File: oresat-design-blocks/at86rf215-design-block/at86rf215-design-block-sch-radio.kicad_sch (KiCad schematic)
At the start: 40 parts, among them J1 SMA, J2 USB4105-GF-A, J3 Conn_01x04, J5 Conn_02x20_Odd_Even, J6 Conn_01x04, J9 Screw_Terminal_01x02, SW1 RESET, U1 AT86RF215, U2 LP2985AIM5-1.8_NOPB, X1 TXETALSANF-26.000000

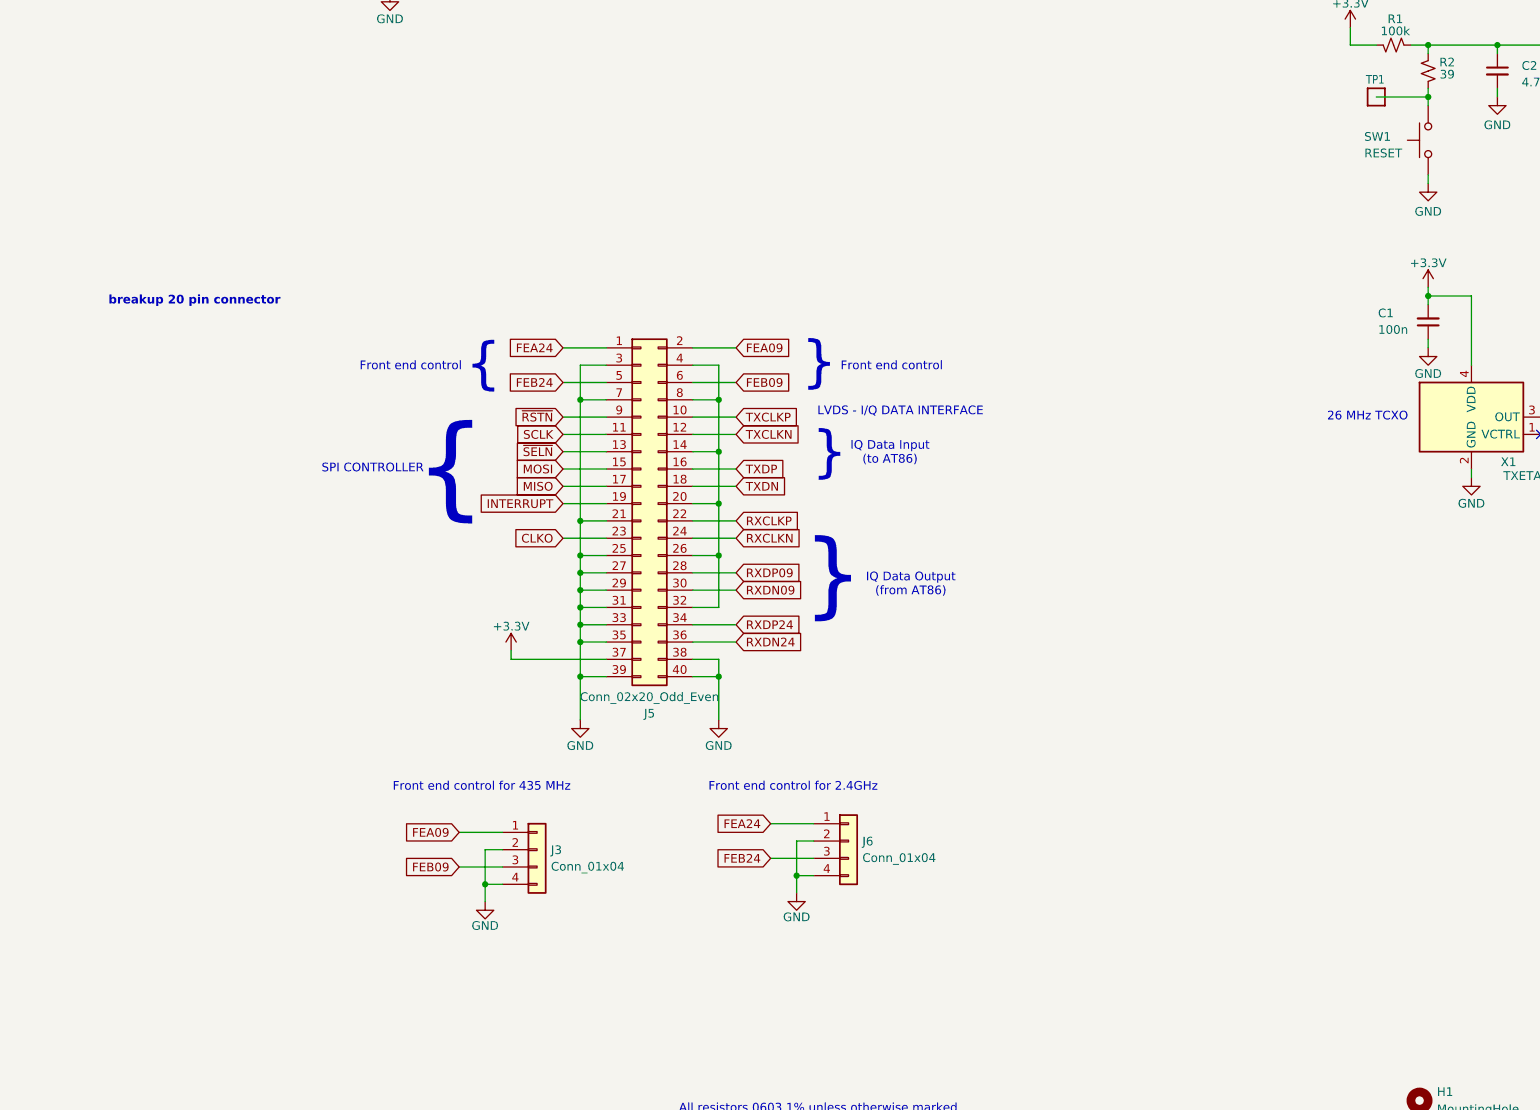
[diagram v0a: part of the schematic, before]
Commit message: more routing progress
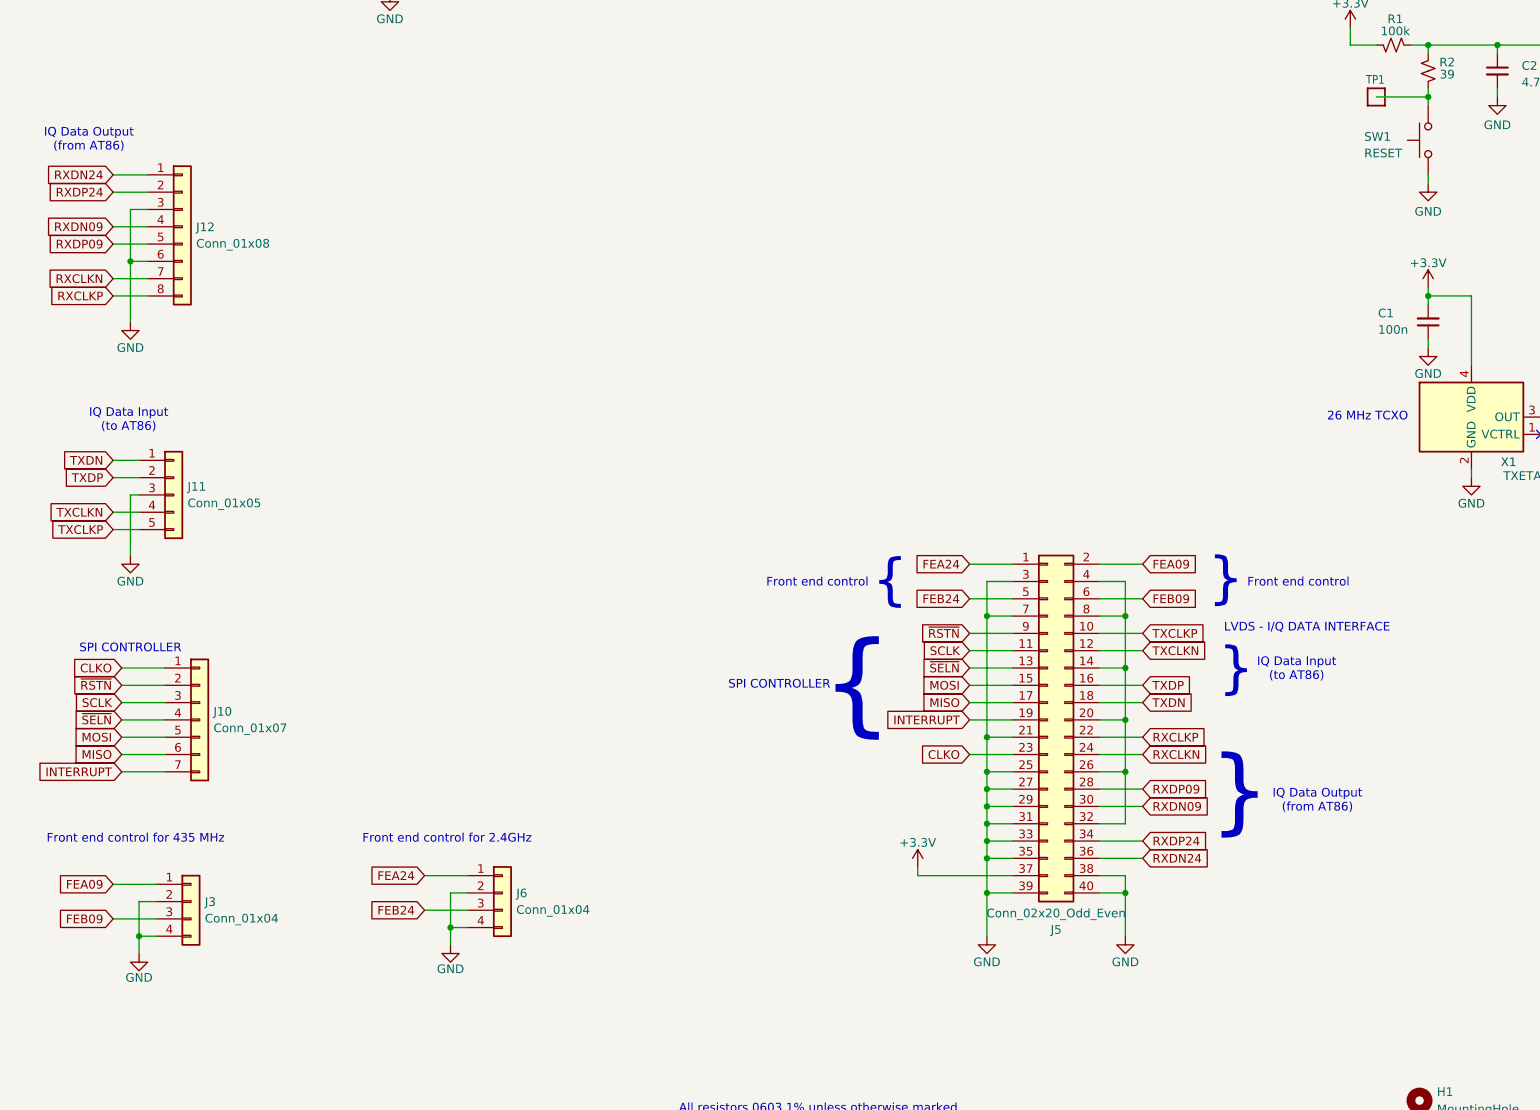
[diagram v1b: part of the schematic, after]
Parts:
- added J10: Conn_01x07, Connector_PinHeader_2.54mm:PinHeader_1x04_P2.54mm_Vertical, symbol Connector_Generic:Conn_01x07
- added J11: Conn_01x05, Connector_PinHeader_2.54mm:PinHeader_1x04_P2.54mm_Vertical, symbol Connector_Generic:Conn_01x05
- added J12: Conn_01x08, Connector_PinHeader_2.54mm:PinHeader_1x04_P2.54mm_Vertical, symbol Connector_Generic:Conn_01x08
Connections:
- net AVSS: now also J11.3 (Pin_3), J12.3 (Pin_3), J12.6 (Pin_6)
- net CLKO: now also J10.1 (Pin_1)
- net INTERRUPT: now also J10.7 (Pin_7)
- net MISO: now also J10.6 (Pin_6)
- net MOSI: now also J10.5 (Pin_5)
- net RXCLKN: now also J12.7 (Pin_7)
- net RXCLKP: now also J12.8 (Pin_8)
- net RXDN09: now also J12.4 (Pin_4)
- net RXDN24: now also J12.1 (Pin_1)
- net RXDP09: now also J12.5 (Pin_5)
- net RXDP24: now also J12.2 (Pin_2)
- net SCLK: now also J10.3 (Pin_3)
- net TXCLKN: now also J11.4 (Pin_4)
- net TXCLKP: now also J11.5 (Pin_5)
- net TXDN: now also J11.1 (Pin_1)
- net TXDP: now also J11.2 (Pin_2)
- net ~{RSTN}: now also J10.2 (Pin_2)
- net ~{SELN}: now also J10.4 (Pin_4)
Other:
- note removed: "breakup 20 pin connector"
- moved on the sheet: J3, J5, J6
